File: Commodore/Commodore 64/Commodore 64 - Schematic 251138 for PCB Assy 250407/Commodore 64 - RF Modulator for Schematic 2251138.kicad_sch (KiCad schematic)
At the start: 12 parts

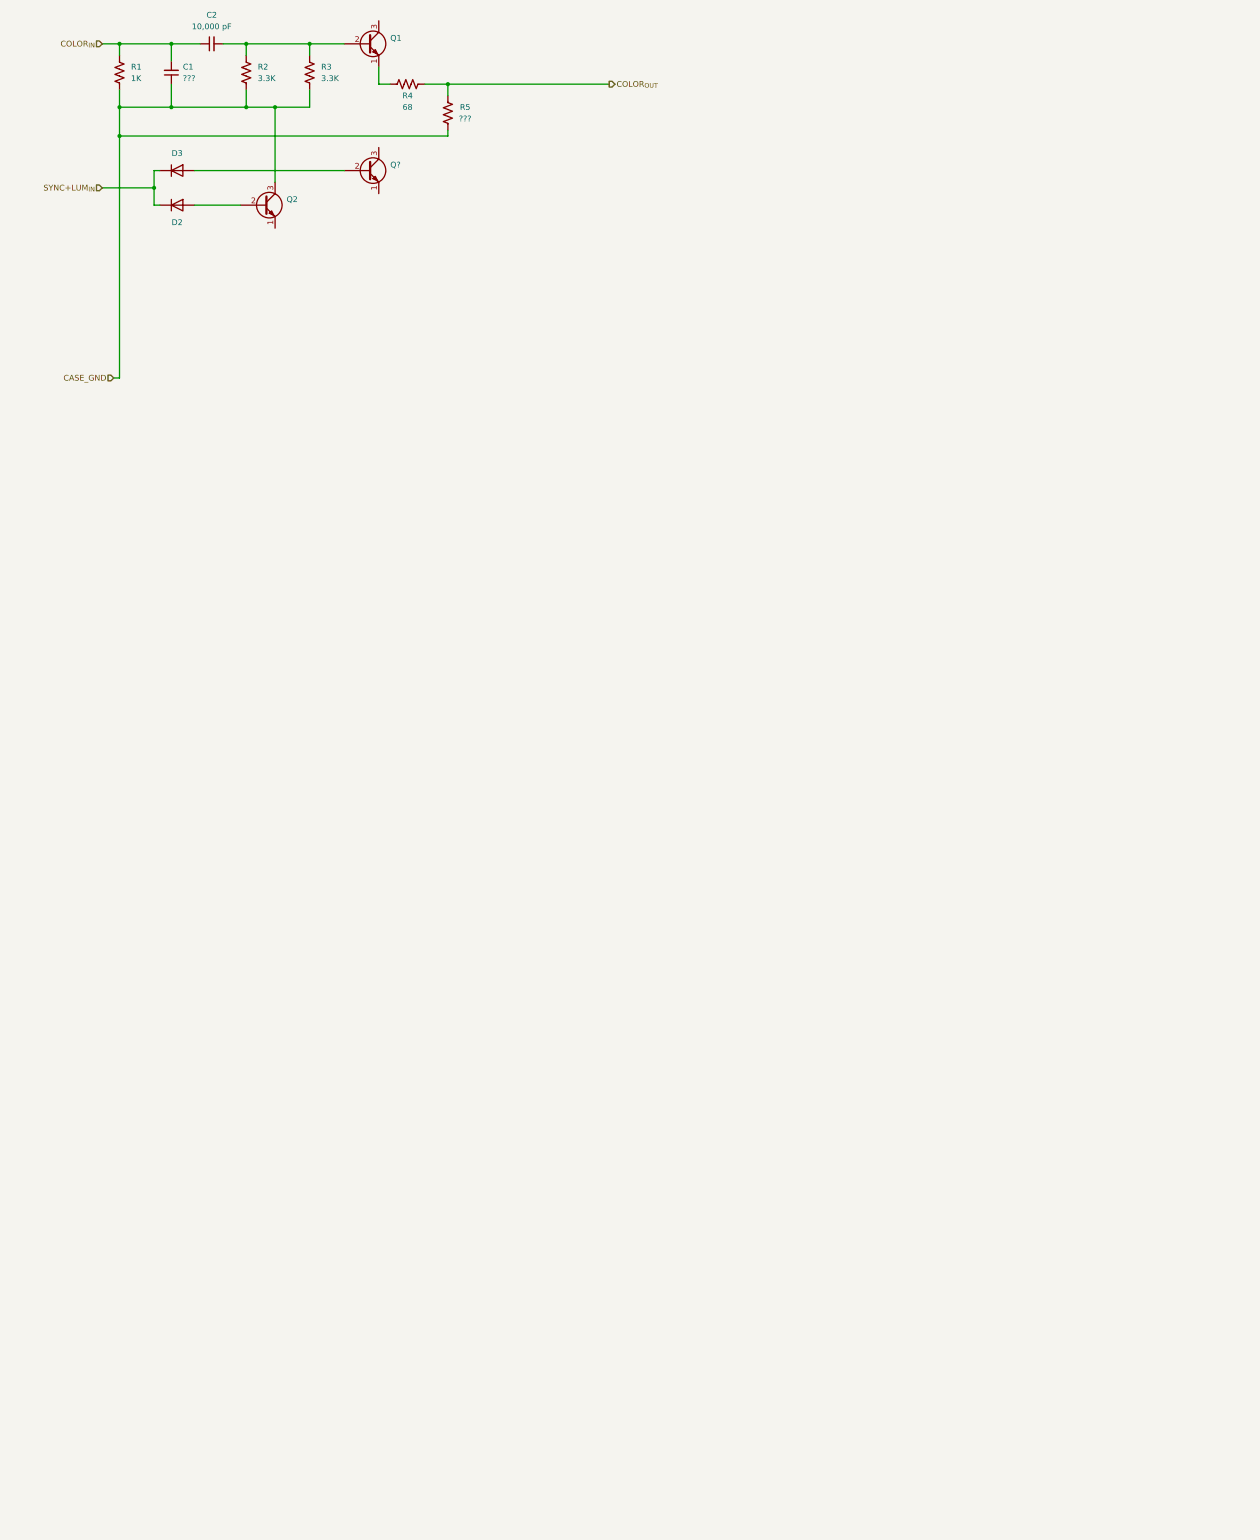
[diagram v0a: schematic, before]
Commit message: Completed C64 Schematic 251138
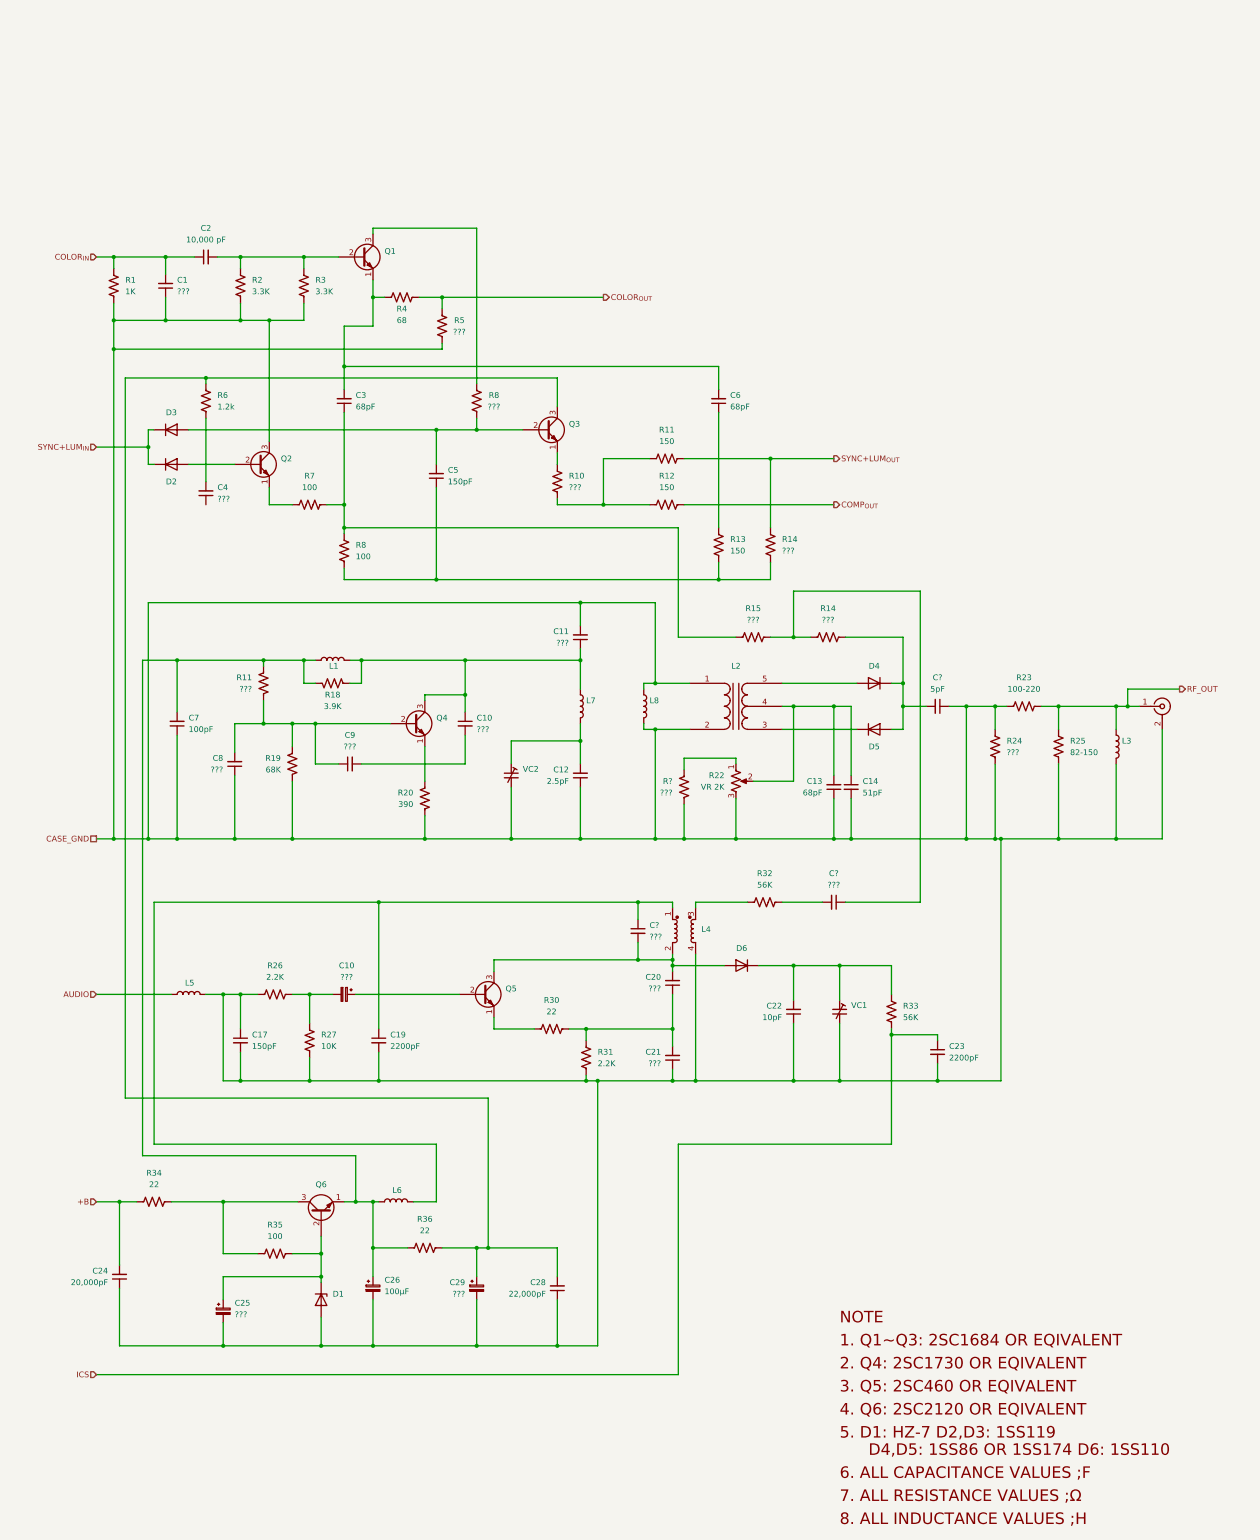
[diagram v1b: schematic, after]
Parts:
- added C10, C25, C29: ???, symbol Device:C_Polarized_Small
- added C10, C11, C20, C21, C4, C8, C9, C? (x2): ???, symbol Device:C_Small
- added C12: 2.5pF, symbol Device:C_Small
- added C13, C3, C6: 68pF, symbol Device:C_Small
- added C14: 51pF, symbol Device:C_Small
- added C17, C5: 150pF, symbol Device:C_Small
- added C19, C23: 2200pF, symbol Device:C_Small
- added C22: 10pF, symbol Device:C_Small
- added C24: 20,000pF, symbol Device:C_Small
- added C26: 100µF, symbol Device:C_Polarized_Small
- added C28: 22,000pF, symbol Device:C_Small
- added C7: 100pF, symbol Device:C_Small
- added C?: 5pF, symbol Device:C_Small
- added D1: D_Zener, symbol Device:D_Zener
- added D4, D5, D6: D, symbol Device:D
- added J?: Conn_Coaxial, symbol Connector:Conn_Coaxial
- added L1, L3, L5, L6, L7, L8: L, symbol Device:L
- added L2: Transformer_1P_SS, symbol Device:Transformer_1P_SS
- added L4: L_Coupled, symbol Device:L_Coupled
- added N?: SHEET_RF_MOD_NOTES, symbol Commodore_64_Schematic_251138:SHEET_RF_MOD_NOTES
- added Q4, Q5, Q6: ~, Package_TO_SOT_THT:TO-39-3, symbol Transistor_BJT:2N2219
- added R10, R11, R14 (x2), R15, R24, R8, R?: ???, symbol Device:R_US
- added R11, R12, R13: 150, symbol Device:R_US
- added R18: 3.9K, symbol Device:R_US
- added R19: 68K, symbol Device:R_US
- added R20: 390, symbol Device:R_US
- added R22: VR 2K, symbol Device:R_Potentiometer_US
- added R23: 100-220, symbol Device:R_US
- added R25: 82-150, symbol Device:R_US
- added R26, R31: 2.2K, symbol Device:R_US
- added R27: 10K, symbol Device:R_US
- added R30, R34, R36: 22, symbol Device:R_US
- added R32, R33: 56K, symbol Device:R_US
- added R35, R7, R8: 100, symbol Device:R_US
- added R6: 1.2k, symbol Device:R_US
- added VC1, VC2: C_Trim_Small, symbol Device:C_Trim_Small
- gave numbers to parts that had none: 1
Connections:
- net CASE_GND: now also C11.2, C12.1, C13.1, C14.2, C17.1, C17.2, C19.2, C21.1, C22.1, C23.2, C24.1, C25.2, C26.2, C28.1, C29.2, C7.1, C8.1, C?.1, D1.2 (A), J?.2 (Ext), L2.1 (AA), L2.2 (AB), L3.2, L4.4, L5.2, L8.1, L8.2, R19.1, R20.1, R22.3, R23.2, R24.1, R24.2, R25.2, R26.1, R27.1, R31.1, R?.1, VC1.2, VC2.2
- net at Q2.1 (E): now also R7.1
- net at Q3.1 (E): now also R10.2
- net at D3.2 (A), Q3.2 (B): now also C5.2, R8.1
- net at Q3.3 (C): now also C28.2, C29.1, R36.1, R6.1
- net at Q1.1 (E), R4.1: now also C3.2, C6.2
- net at Q1.3 (C): now also R8.2
- new net: C12.2, L7.2, VC2.1
- new net: C13.2, C14.1, L2.4 (SC), R22.2
- new net: C19.1, C?.1, L4.1, L6.2
- new net: C20.2, C?.2, D6.2 (A), L4.2, Q5.3 (C)
- new net: R22.1, R?.2
- new net: C4.2, R6.2
- new net: C22.2, D6.1 (K), R33.1, VC1.1
- new net: C26.1, C7.2, L1.1, L6.1, Q6.1 (E), R11.2, R18.2, R36.2
- new net: C25.1, D1.1 (K), Q6.2 (B), R35.1
- new net: Q6.3 (C), R34.1, R35.2
- new net: R10.1, R11.1, R12.2
- new net: Q4.1 (E), R20.2
- new net: C3.1, R15.2, R7.2, R8.2
- new net: C?.2, R32.1
- new net: L4.3, R32.2
- new net: C8.2, C9.1, Q4.2 (B), R11.1, R19.2
- new net: C10.2, C9.2
- new net: C20.1, C21.2, R30.2, R31.2
- new net: C10.1, C11.1, L1.2, L7.1, Q4.3 (C), R18.1
- new net: Q5.1 (E), R30.1
- new net: C?.1, R14.2, R15.1
- new net: C?.2, D4.1 (K), D5.2 (A), R14.1
- new net: C5.1, R13.1, R14.1, R8.1
- new net: C10.1, Q5.2 (B)
- new net: C10.2, R26.2, R27.2
- new net: C6.1, R13.2
- new net: D4.2 (A), L2.5 (SB)
- new net: D5.1 (K), L2.3 (SA)
- new net +B: C24.2, R34.2
- new net AUDIO: L5.1
- new net COMP_{OUT}: R12.1
- new net ICS: C23.1, R33.2
- new net RF_OUT: J?.1 (In), L3.1, R23.1, R25.1
- new net SYNC+LUM_{OUT}: R11.2, R14.2
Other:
- moved on the sheet: C1, C2, D2, D3, Q1, Q2, Q3, R1, R2, R3, R4, R5
